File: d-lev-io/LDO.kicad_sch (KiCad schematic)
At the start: 7 parts, among them U1 AP1117-ADJ

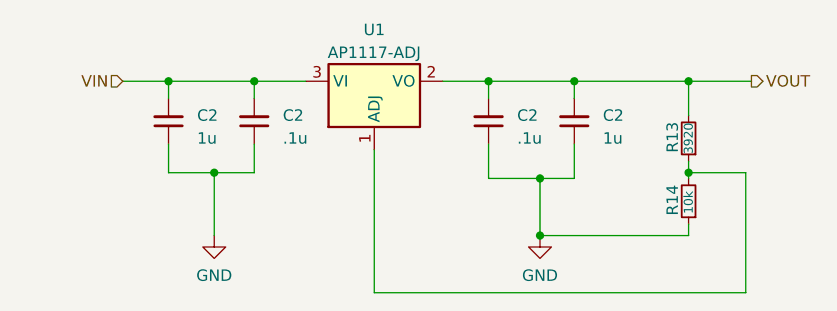
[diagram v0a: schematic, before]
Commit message: many many changes'
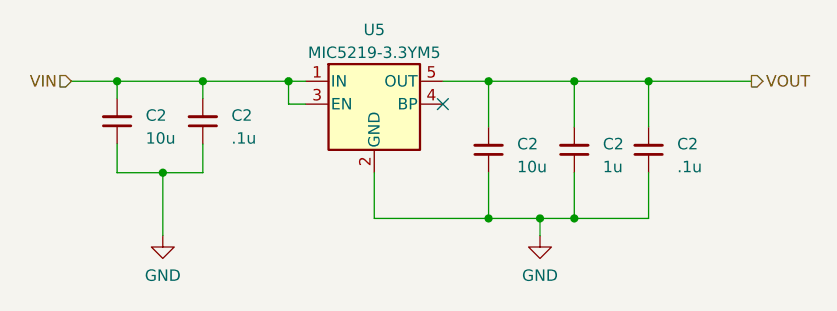
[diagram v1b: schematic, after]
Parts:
- removed R13: 3920, Resistor_SMD:R_0805_2012Metric_Pad1.20x1.40mm_HandSolder, symbol Device:R_Small
- removed R14: 10k, Resistor_SMD:R_0805_2012Metric_Pad1.20x1.40mm_HandSolder, symbol Device:R_Small
- removed U1: AP1117-ADJ, Package_TO_SOT_SMD:SOT-223-3_TabPin2, symbol Regulator_Linear:AP1117-ADJ
- added C2: 10u, symbol Device:C_Small
- added U5: MIC5219-3.3YM5, Package_TO_SOT_SMD:SOT-23-5, symbol Regulator_Linear:MIC5219-3.3YM5
- C2: value 1u -> 10u
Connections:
- net GND: now also C2.1, U5.2 (GND)
- net VIN: now also U5.1 (IN), U5.3 (EN)
- net VOUT: now also C2.2, U5.5 (OUT)
- no-connect marks 0 -> 1
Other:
- moved on the sheet: C2
